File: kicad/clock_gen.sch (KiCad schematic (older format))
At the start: 20 parts, among them J1 Programming, SW1 Rotary_Encoder, SW2 Rotary_Encoder, U1 MachXO2-1200-QFN32, U2 LM3480-3.3, U3 74HCT541, X1 DSC1001AE5-001.2000

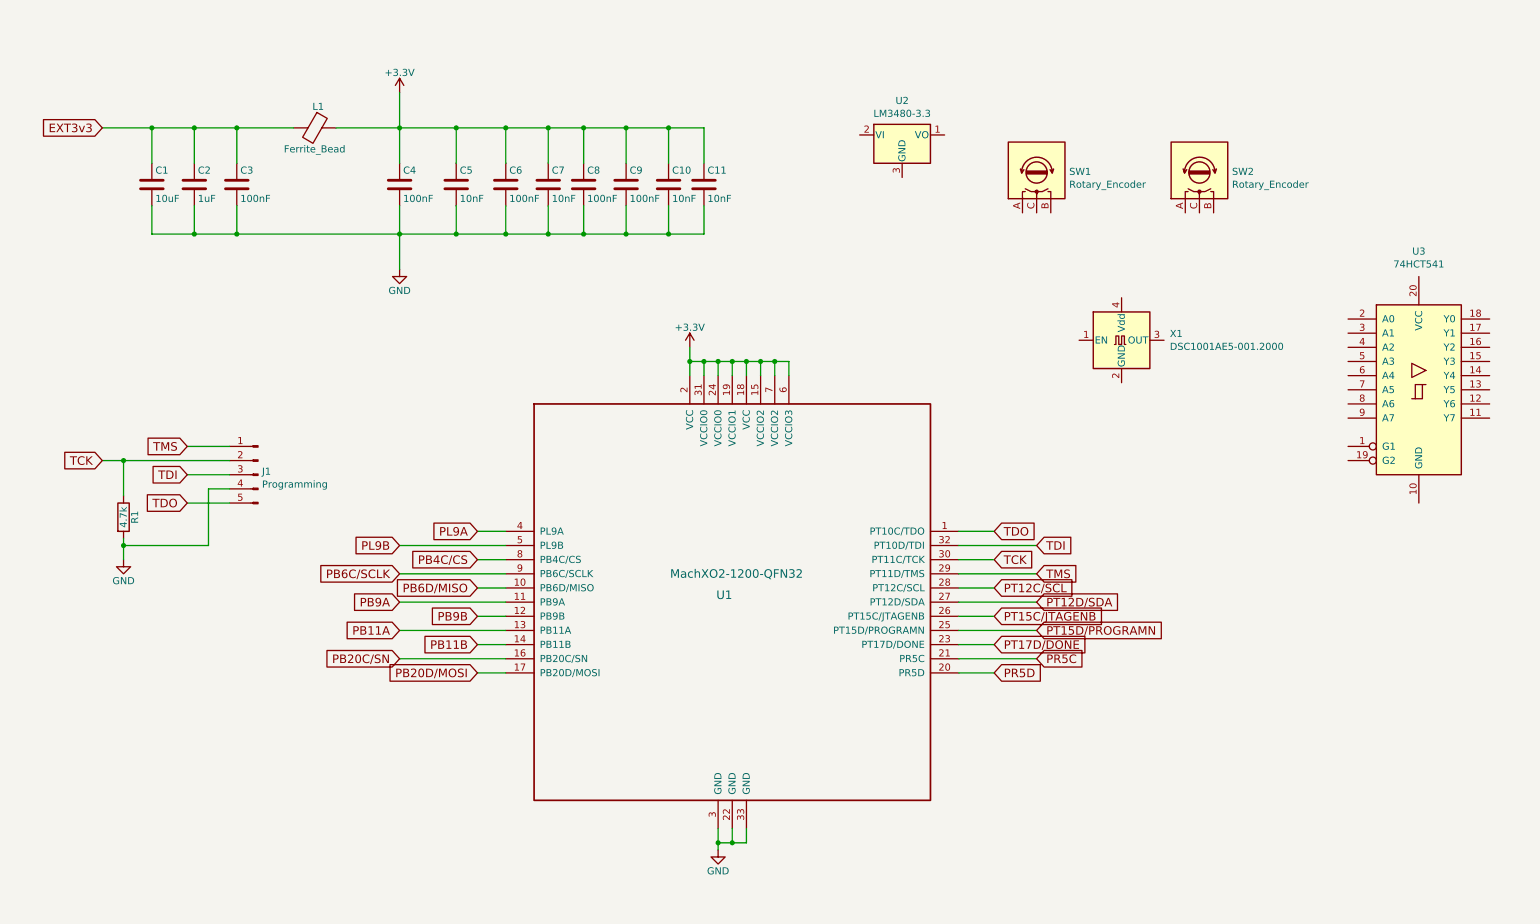
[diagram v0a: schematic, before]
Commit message: Finished PCB
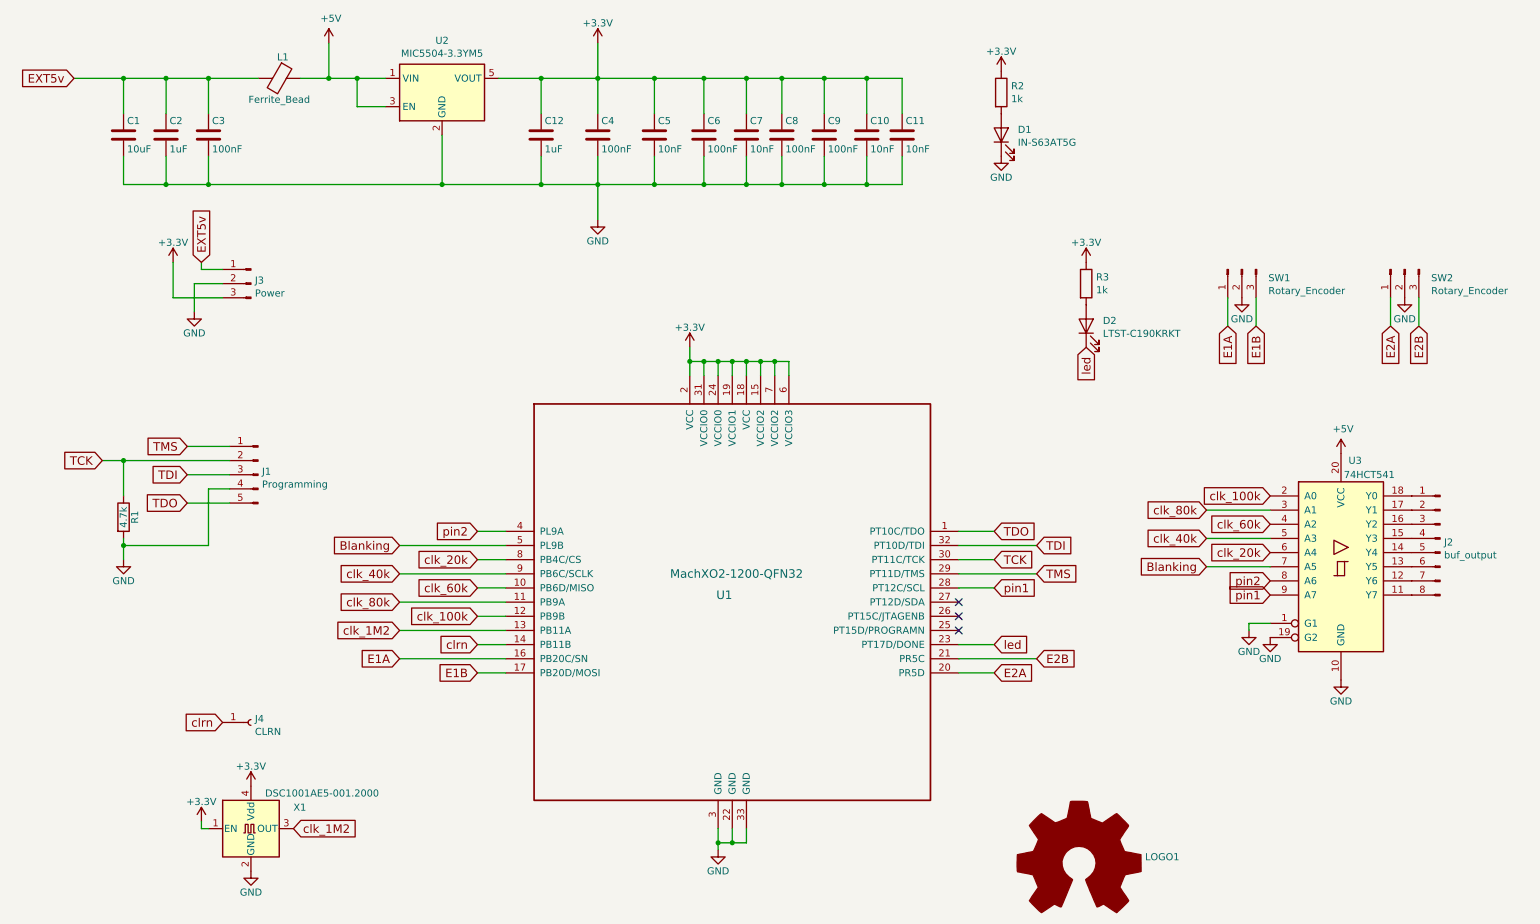
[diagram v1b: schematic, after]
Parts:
- removed SW1, SW2: Rotary_Encoder, Potentiometer_THT:Potentiometer_Bourns_PTV09A-2_Single_Horizontal, symbol Device:Rotary_Encoder
- removed U2: LM3480-3.3, Package_TO_SOT_SMD:SOT-23, symbol Regulator_Linear:LM3480-3.3
- added C12: 1uF, Capacitor_SMD:C_0603_1608Metric, symbol Device:C
- added D1: IN-S63AT5G, LED_SMD:LED_0603_1608Metric, symbol Device:LED
- added D2: LTST-C190KRKT, LED_SMD:LED_0603_1608Metric, symbol Device:LED
- added J2: buf_output, Connector_PinHeader_1.27mm:PinHeader_1x08_P1.27mm_Vertical, symbol Connector:Conn_01x08_Male
- added J3: Power, Connector_PinHeader_1.27mm:PinHeader_1x03_P1.27mm_Vertical, symbol Connector:Conn_01x03_Male
- added J4: CLRN, Connector_PinHeader_1.27mm:PinHeader_1x01_P1.27mm_Vertical, symbol Connector:Conn_01x01_Female
- added LOGO1: Logo_Open_Hardware_Large, logo:clk, symbol Graphic:Logo_Open_Hardware_Large
- added R2, R3: 1k, Resistor_SMD:R_0603_1608Metric, symbol Device:R
- added SW1, SW2: Rotary_Encoder, Connector_PinHeader_1.27mm:PinHeader_1x03_P1.27mm_Vertical, symbol Connector:Conn_01x03_Male
- added U2: MIC5504-3.3YM5, Package_TO_SOT_SMD:SOT-23-5, symbol Regulator_Linear:MIC5504-3.3YM5
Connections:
- net PB11A is gone; now on net clk_1M2: U1.13 (PB11A)
- net PB4C/CS is gone; now on net clk_20k: U1.8 (PB4C/CS)
- net PB6C/SCLK is gone; now on net clk_40k: U1.9 (PB6C/SCLK)
- net PB6D/MISO is gone; now on net clk_60k: U1.10 (PB6D/MISO)
- net PB9A is gone; now on net clk_80k: U1.11 (PB9A)
- net PB9B is gone; now on net clk_100k: U1.12 (PB9B)
- net PL9A is gone; now on net pin2: U1.4 (PL9A)
- net PL9B is gone; now on net Blanking: U1.5 (PL9B)
- net PT12C/SCL is gone; now on net pin1: U1.28 (PT12C/SCL)
- net +3V3: now also X1.1 (EN), X1.4 (Vdd), C12.1, J3.3 (Pin_3), R2.1, R3.1, U2.5 (VOUT); no longer L1.1
- net GND: now also U3.1 (G1), U3.10 (GND), U3.19 (G2), X1.2 (GND), C12.2, D1.1 (K), J3.2 (Pin_2), SW1.2 (Pin_2), SW2.2 (Pin_2), U2.2 (GND)
- net clk_1M2: now reaches X1.3 (OUT)
- net at U3.11 (Y7): now also J2.8 (Pin_8)
- net at U3.12 (Y6): now also J2.7 (Pin_7)
- net at U3.13 (Y5): now also J2.6 (Pin_6)
- net at U3.14 (Y4): now also J2.5 (Pin_5)
- net at U3.15 (Y3): now also J2.4 (Pin_4)
- net at U3.16 (Y2): now also J2.3 (Pin_3)
- net at U3.17 (Y1): now also J2.2 (Pin_2)
- net at U3.18 (Y0): now also J2.1 (Pin_1)
- net clk_100k: now reaches U3.2 (A0)
- net +5V: now reaches U3.20 (VCC)
- net +5V: now also L1.1, U2.1 (VIN), U2.3 (EN)
- net clk_80k: now reaches U3.3 (A1)
- net clk_60k: now reaches U3.4 (A2)
- net clk_40k: now reaches U3.5 (A3)
- net clk_20k: now reaches U3.6 (A4)
- net Blanking: now reaches U3.7 (A5)
- net pin2: now reaches U3.8 (A6)
- net pin1: now reaches U3.9 (A7)
- net EXT3v3 renamed EXT5v
- net EXT5v: now also J3.1 (Pin_1)
- net PB11B renamed clrn
- net clrn: now also J4.1 (Pin_1)
- net PB20C/SN renamed E1A
- net E1A: now also SW1.1 (Pin_1)
- net PB20D/MOSI renamed E1B
- net E1B: now also SW1.3 (Pin_3)
- net PR5C renamed E2B
- net E2B: now also SW2.3 (Pin_3)
- net PR5D renamed E2A
- net E2A: now also SW2.1 (Pin_1)
- net PT12D/SDA: no longer names the net of U1.27 (PT12D/SDA)
- net PT15C/JTAGENB: no longer names the net of U1.26 (PT15C/JTAGENB)
- net PT15D/PROGRAMN: no longer names the net of U1.25 (PT15D/PROGRAMN)
- net PT17D/DONE renamed led
- net led: now also D2.1 (K)
- new net: D1.2 (A), R2.2
- new net: D2.2 (A), R3.2
- no-connect marks 0 -> 3
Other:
- moved on the sheet: C1, C10, C11, C2, C3, C4, C5, C6, C7, C8, C9, L1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
